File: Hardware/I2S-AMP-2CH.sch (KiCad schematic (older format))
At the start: 21 parts, among them U4 TAS5760MDCAR

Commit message: various fixes
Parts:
- removed C32: 100n, Capacitor_SMD:C_0603_1608Metric_Pad1.08x0.95mm_HandSolder, symbol dsp-amplifier-x4-rescue:Capacitor
- removed C36, C37: 4.7u, Capacitor_SMD:C_0805_2012Metric_Pad1.18x1.45mm_HandSolder, symbol dsp-amplifier-x4-rescue:Capacitor
- removed U4: TAS5760MDCAR, AMPx2 _footprints:HTSSOP-48, symbol dsp-amplifier-x4-rescue:TAS5760MDCAR
- added C32: 470u, Capacitor_THT:CP_Radial_D14.0mm_P5.00mm, symbol Device:CP
- added U?1: TAS5760MDCAR, Package_SO:HTSSOP-32-1EP_6.1x11mm_P0.65mm_EP5.2x11mm_Mask4.11x4.36mm_ThermalVias, symbol tas5760:TAS5760MDCAR
- C25: value 1u -> 100n; Mfr.Nr. GRM188R71C105KE15D -> GRM188R71H104KA93D
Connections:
- net labels added: FREQ, PBTL
- wire segments 107 -> 100
- no-connect marks 14 -> 0

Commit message: started routing
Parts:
- removed C35: 220n, Capacitor_SMD:C_0603_1608Metric_Pad1.08x0.95mm_HandSolder, symbol dsp-amplifier-x4-rescue:Capacitor
- removed C38, C40, C41: 680n, Capacitor_SMD:C_0603_1608Metric_Pad1.08x0.95mm_HandSolder, symbol dsp-amplifier-x4-rescue:Capacitor
- removed L2, L3, L4: 10u, Capacitor_SMD:C_0805_2012Metric_Pad1.18x1.45mm_HandSolder, symbol dsp-amplifier-x4-rescue:Inductor
- added C56: 220n, Capacitor_SMD:C_0603_1608Metric_Pad1.08x0.95mm_HandSolder, symbol Device:C
- added C59, C60, C61: 680n, Capacitor_SMD:C_0603_1608Metric_Pad1.08x0.95mm_HandSolder, symbol Device:C
- added L4, L5, L6: 10u, Inductor_SMD:L_Abracon_ASPI-0630LR, symbol Device:L
- C48: renamed from C26; footprint Capacitor_SMD:C_0603_1608Metric_Pad1.08x0.95mm_HandSolder -> Capacitor_SMD:C_0805_2012Metric_Pad1.18x1.45mm_HandSolder; symbol dsp-amplifier-x4-rescue:Capacitor -> Device:C
- C49: renamed from C27; footprint Capacitor_SMD:C_0603_1608Metric_Pad1.08x0.95mm_HandSolder -> Capacitor_SMD:C_0805_2012Metric_Pad1.18x1.45mm_HandSolder; symbol dsp-amplifier-x4-rescue:Capacitor -> Device:C
- C50: renamed from C30; footprint Capacitor_SMD:C_0603_1608Metric_Pad1.08x0.95mm_HandSolder -> Capacitor_SMD:C_0805_2012Metric_Pad1.18x1.45mm_HandSolder; symbol dsp-amplifier-x4-rescue:Capacitor -> Device:C
- C51: renamed from C25; symbol dsp-amplifier-x4-rescue:Capacitor -> Device:C
- C52: renamed from C31; symbol dsp-amplifier-x4-rescue:Capacitor -> Device:C
- C53: renamed from C32; footprint Capacitor_THT:CP_Radial_D14.0mm_P5.00mm -> Capacitor_THT:CP_Radial_D16.0mm_P7.50mm
- C54: renamed from C34; symbol dsp-amplifier-x4-rescue:Capacitor -> Device:C
- C55: renamed from C29; symbol dsp-amplifier-x4-rescue:Capacitor -> Device:C
- C57: renamed from C33; symbol dsp-amplifier-x4-rescue:Capacitor -> Device:C
- C58: renamed from C39; symbol dsp-amplifier-x4-rescue:Capacitor -> Device:C
- L3: renamed from L1; footprint Capacitor_SMD:C_0805_2012Metric_Pad1.18x1.45mm_HandSolder -> Inductor_SMD:L_Abracon_ASPI-0630LR; symbol dsp-amplifier-x4-rescue:Inductor -> Device:L
- renumbered U?1 to U6
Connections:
- wire segments 100 -> 106

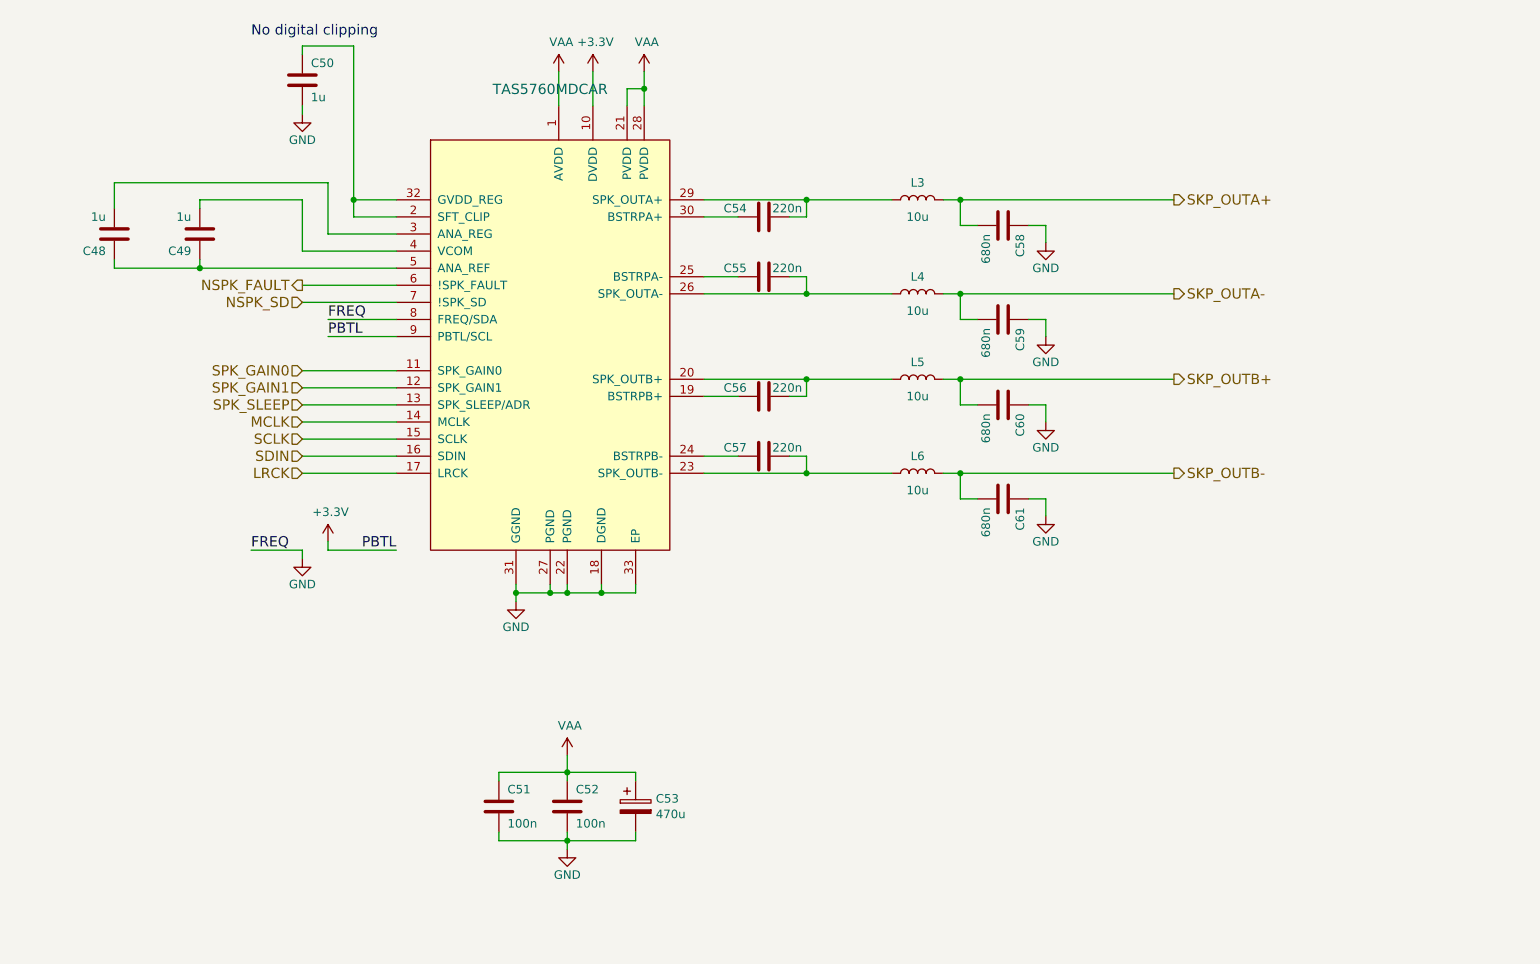
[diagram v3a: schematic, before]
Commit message: bugfixes, made smaller
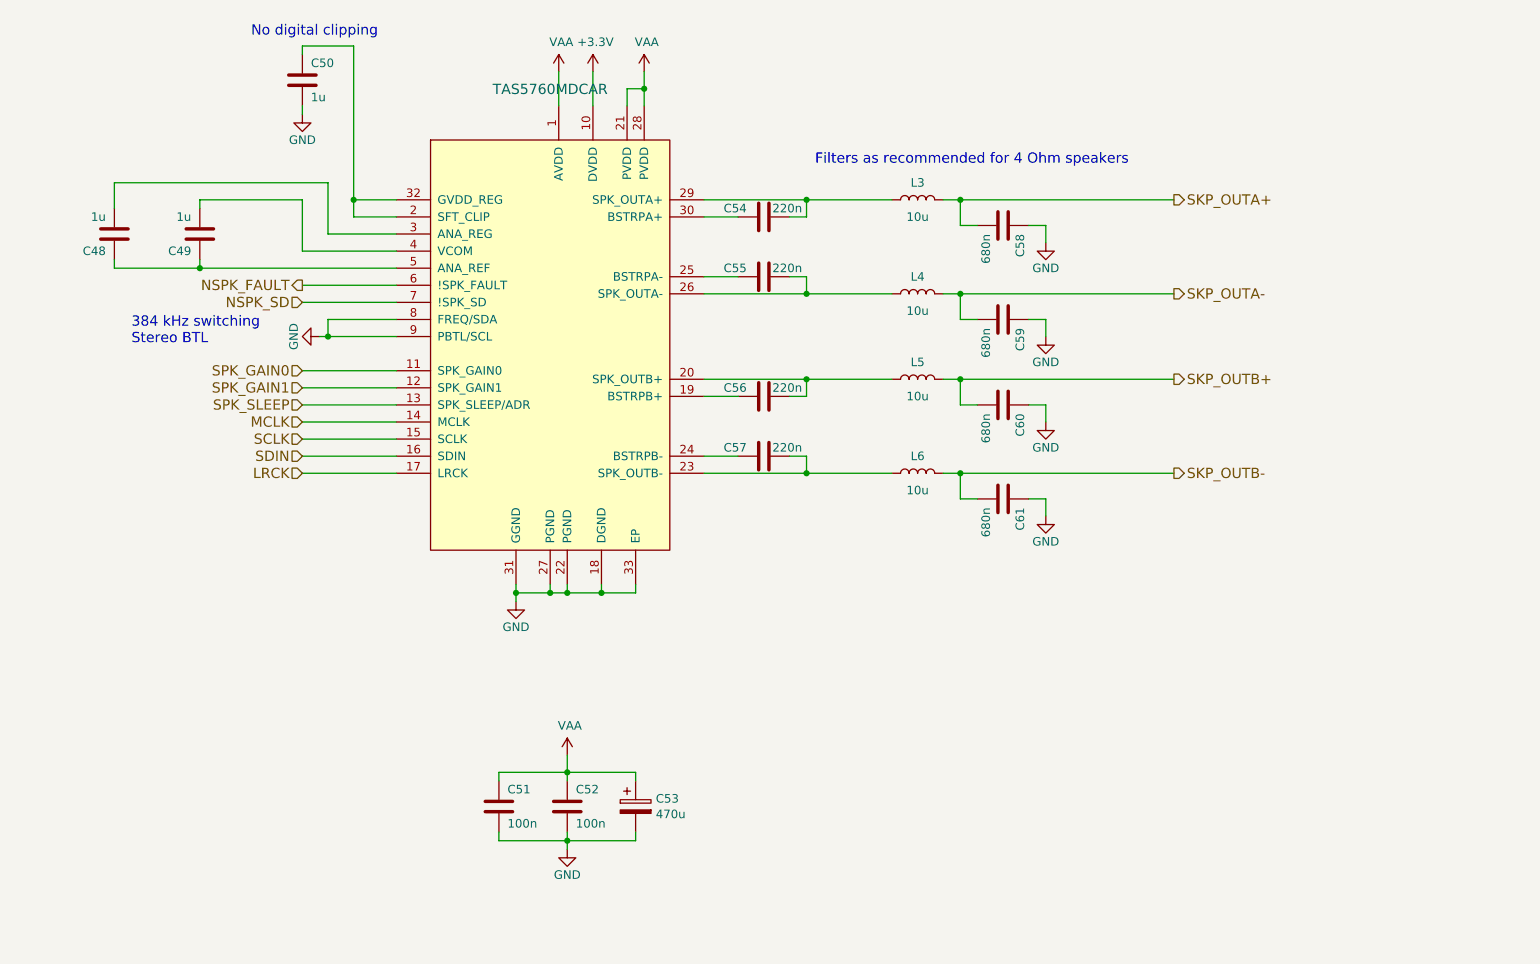
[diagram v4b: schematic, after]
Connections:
- net +3V3: no longer U6.9 (PBTL/SCL)
- net GND: now also U6.9 (PBTL/SCL)
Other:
- note added: "384 kHz switching\nStereo BTL"
- note added: "Filters as recommended for 4 Ohm speakers"
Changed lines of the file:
@@
 	0    -1   -1   0
-$EndComp
-$Comp
-L power:GND #PWR073
-U 1 1 5750BB5F
-P 2950 4450
-AR Path="/5AF9FF80/5750BB5F" Ref="#PWR073"  Part="1"
-AR Path="/608A6138/5750BB5F" Ref="#PWR086"  Part="1"
-F 0 "#PWR086" H 2950 4200 50  0001 C CNN
-F 1 "GND" H 2950 4300 50  0000 C CNN
-F 2 "" H 2950 4450 50  0000 C CNN
-F 3 "" H 2950 4450 50  0000 C CNN
-	1    2950 4450
-	1    0    0    -1
 $EndComp
 Wire Wire Line
@@
 Wire Wire Line
 	4500 5600 4500 5700
-$Comp
-L power:+3.3V #PWR?
-U 1 1 60734777
-P 3100 4350
-AR Path="/60734777" Ref="#PWR?"  Part="1"
-AR Path="/5AF9FF80/60734777" Ref="#PWR074"  Part="1"
-AR Path="/608A6138/60734777" Ref="#PWR087"  Part="1"
-F 0 "#PWR087" H 3100 4200 50  0001 C CNN
-F 1 "+3.3V" H 3115 4523 50  0000 C CNN
-F 2 "" H 3100 4350 50  0001 C CNN
-F 3 "" H 3100 4350 50  0001 C CNN
-	1    3100 4350
-	1    0    0    -1
-$EndComp
 $Comp
 L power:VAA #PWR077
@@
 Wire Wire Line
 	2950 1450 3250 1450
-Text Label 3100 3050 0    60   ~ 0
-FREQ
-Text Label 3100 3150 0    60   ~ 0
-PBTL
 Wire Wire Line
 	3100 3050 3500 3050
-Wire Wire Line
-	3500 3150 3100 3150
-Text Label 2650 4400 0    60   ~ 0
-FREQ
-Text Label 3500 4400 2    60   ~ 0
-PBTL
-Wire Wire Line
-	3500 4400 3100 4400
-Wire Wire Line
-	3100 4350 3100 4400
-Wire Wire Line
-	2950 4450 2950 4400
-Wire Wire Line
-	2950 4400 2650 4400
 $Comp
 L power:+3.3V #PWR?
@@
 Wire Wire Line
 	4100 6050 4100 6100
-$Comp
-L tas5760:TAS5760MDCAR U6
-U 1 1 608A7BF7
-P 4400 3200
-AR Path="/5AF9FF80/608A7BF7" Ref="U6"  Part="1"
-AR Path="/608A6138/608A7BF7" Ref="U7"  Part="1"
-F 0 "U6" H 4400 5150 60  0001 C TNN
-F 1 "TAS5760MDCAR" H 4400 4697 60  0000 C CNN
-F 2 "Package_SO:HTSSOP-32-1EP_6.1x11mm_P0.65mm_EP5.2x11mm_Mask4.11x4.36mm_ThermalVias" H 4300 3100 60  0001 C CNN
-F 3 "" H 4400 3200 60  0000 C CNN
-	1    4400 3200
-	1    0    0    -1
-$EndComp
 Wire Wire Line
 	5300 3950 5900 3950
@@
 	4900 4650 4900 4600
 Connection ~ 4700 4650
+$Comp
+L power:GND #PWR0122
+U 1 1 60B105F1
+P 3050 3150
+AR Path="/5AF9FF80/60B105F1" Ref="#PWR0122"  Part="1"
+AR Path="/608A6138/60B105F1" Ref="#PWR0124"  Part="1"
+F 0 "#PWR0124" H 3050 2900 50  0001 C CNN
+F 1 "GND" H 3050 3000 50  0000 C CNN
+F 2 "" H 3050 3150 50  0000 C CNN
+F 3 "" H 3050 3150 50  0000 C CNN
+	1    3050 3150
+	0    1    1    0
+$EndComp
+$Comp
+L tas5760:TAS5760MDCAR U6
+U 1 1 608A7BF7
+P 4400 3200
+AR Path="/5AF9FF80/608A7BF7" Ref="U6"  Part="1"
+AR Path="/608A6138/608A7BF7" Ref="U7"  Part="1"
+F 0 "U6" H 4400 5150 60  0001 C TNN
+F 1 "TAS5760MDCAR" H 4400 4697 60  0000 C CNN
+F 2 "Package_SO:HTSSOP-32-1EP_6.1x11mm_P0.65mm_EP5.2x11mm_Mask4.11x4.36mm_ThermalVias" H 4300 3100 60  0001 C CNN
+F 3 "" H 4400 3200 60  0000 C CNN
+	1    4400 3200
+	1    0    0    -1
+$EndComp
+Wire Wire Line
+	3050 3150 3100 3150
+Wire Wire Line
+	3100 3050 3100 3150
+Connection ~ 3100 3150
+Wire Wire Line
+	3100 3150 3500 3150
+Text Notes 5950 2150 0    60   ~ 0
+Filters as recommended for 4 Ohm speakers
+Text Notes 1950 3200 0    60   ~ 0
+384 kHz switching\nStereo BTL
 $EndSCHEMATC

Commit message: style fixes, spi/i2c
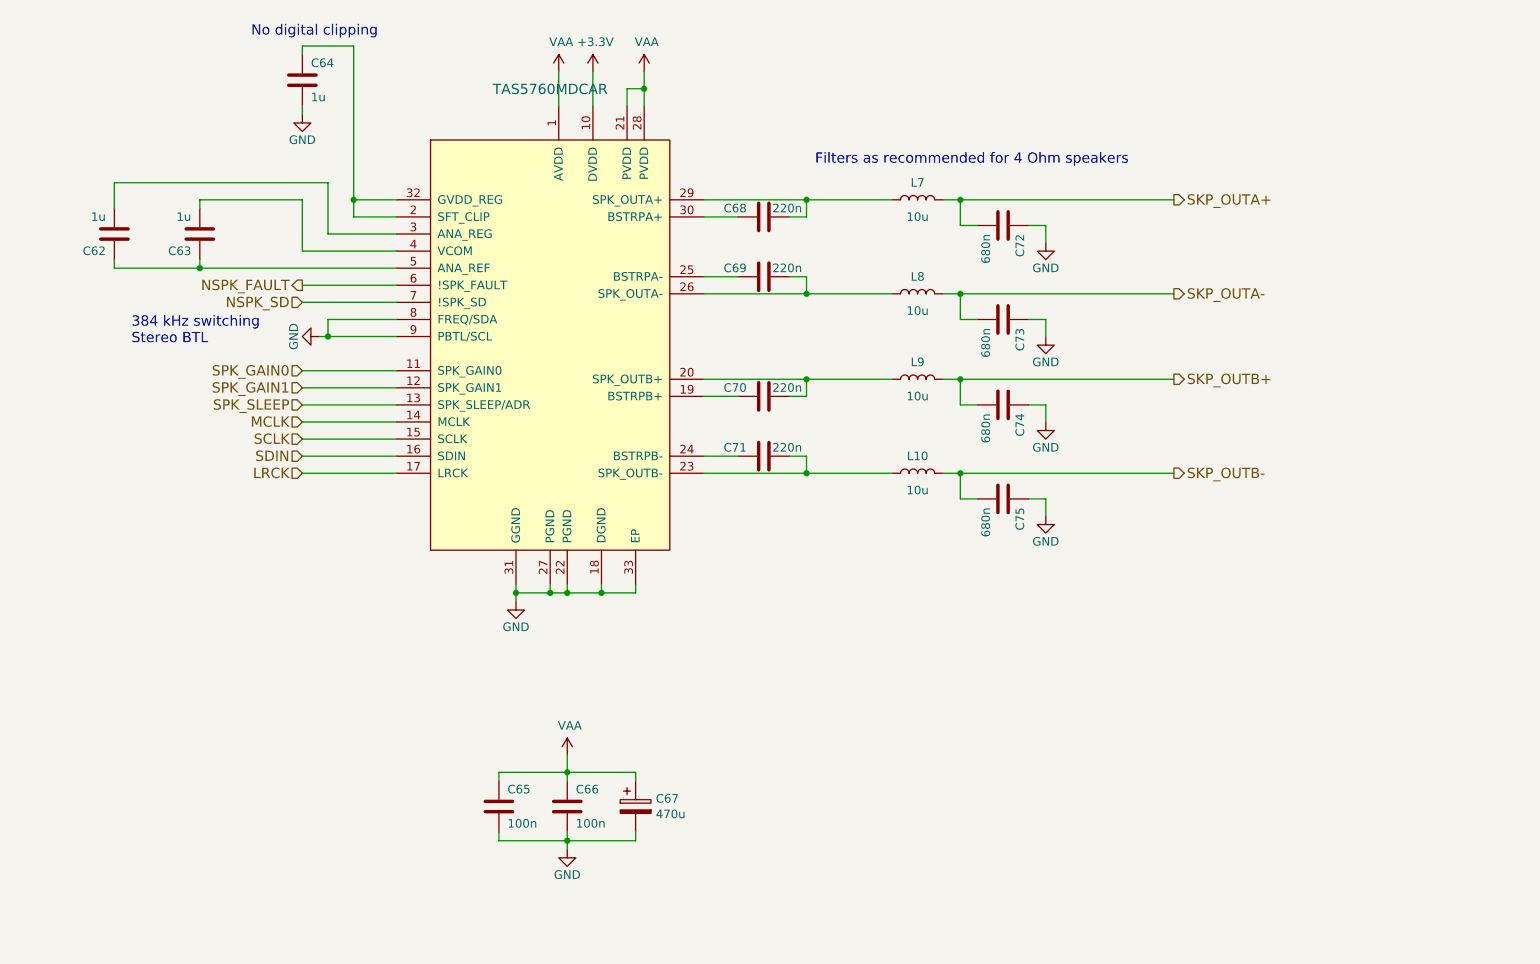
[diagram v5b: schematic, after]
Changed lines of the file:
@@
 AR Path="/5AF9FF80/574C11BE" Ref="C50"  Part="1"
 AR Path="/608A6138/574C11BE" Ref="C64"  Part="1"
-F 0 "C50" H 3000 1750 50  0000 L CNN
+F 0 "C64" H 3000 1750 50  0000 L CNN
 F 1 "1u" H 3000 1550 50  0000 L CNN
 F 2 "Capacitor_SMD:C_0805_2012Metric_Pad1.18x1.45mm_HandSolder" V 2650 1790 50  0001 C CNN
@@
 AR Path="/5AF9FF80/5B067CFE" Ref="C49"  Part="1"
 AR Path="/608A6138/5B067CFE" Ref="C63"  Part="1"
-F 0 "C49" H 2400 2650 50  0000 L CNN
+F 0 "C63" H 2400 2650 50  0000 L CNN
 F 1 "1u" H 2400 2450 50  0000 L CNN
 F 2 "Capacitor_SMD:C_0805_2012Metric_Pad1.18x1.45mm_HandSolder" V 2050 2690 50  0001 C CNN
@@
 AR Path="/5AF9FF80/5B067CFF" Ref="C48"  Part="1"
 AR Path="/608A6138/5B067CFF" Ref="C62"  Part="1"
-F 0 "C48" H 1900 2650 50  0000 L CNN
+F 0 "C62" H 1900 2650 50  0000 L CNN
 F 1 "1u" H 1900 2450 50  0000 L CNN
 F 2 "Capacitor_SMD:C_0805_2012Metric_Pad1.18x1.45mm_HandSolder" V 1550 2690 50  0001 C CNN
@@
 AR Path="/5AF9FF80/574C26C6" Ref="C52"  Part="1"
 AR Path="/608A6138/574C26C6" Ref="C66"  Part="1"
-F 0 "C52" H 4550 6000 50  0000 L CNN
+F 0 "C66" H 4550 6000 50  0000 L CNN
 F 1 "100n" H 4550 5800 50  0000 L CNN
 F 2 "Capacitor_SMD:C_0603_1608Metric_Pad1.08x0.95mm_HandSolder" V 4200 6040 50  0001 C CNN
@@
 AR Path="/5AF9FF80/5B067D0D" Ref="C57"  Part="1"
 AR Path="/608A6138/5B067D0D" Ref="C71"  Part="1"
-F 0 "C57" V 5700 3950 50  0000 L CNN
+F 0 "C71" V 5700 3950 50  0000 L CNN
 F 1 "220n" V 5700 3800 50  0000 R CNN
 F 2 "Capacitor_SMD:C_0603_1608Metric_Pad1.08x0.95mm_HandSolder" V 5350 3990 50  0001 C CNN
@@
 AR Path="/5AF9FF80/5B067D11" Ref="C55"  Part="1"
 AR Path="/608A6138/5B067D11" Ref="C69"  Part="1"
-F 0 "C55" V 5700 2900 50  0000 L CNN
+F 0 "C69" V 5700 2900 50  0000 L CNN
 F 1 "220n" V 5700 2750 50  0000 R CNN
 F 2 "Capacitor_SMD:C_0603_1608Metric_Pad1.08x0.95mm_HandSolder" V 5350 2940 50  0001 C CNN
@@
 AR Path="/5AF9FF80/5B067D13" Ref="C54"  Part="1"
 AR Path="/608A6138/5B067D13" Ref="C68"  Part="1"
-F 0 "C54" V 5700 2550 50  0000 L CNN
+F 0 "C68" V 5700 2550 50  0000 L CNN
 F 1 "220n" V 5700 2400 50  0000 R CNN
 F 2 "Capacitor_SMD:C_0603_1608Metric_Pad1.08x0.95mm_HandSolder" V 5350 2590 50  0001 C CNN
@@
 AR Path="/5AF9FF80/6097B2F1" Ref="C53"  Part="1"
 AR Path="/608A6138/6097B2F1" Ref="C67"  Part="1"
-F 0 "C53" H 5018 5946 50  0000 L CNN
+F 0 "C67" H 5018 5946 50  0000 L CNN
 F 1 "470u" H 5018 5855 50  0000 L CNN
 F 2 "Capacitor_THT:CP_Radial_D16.0mm_P7.50mm" H 4938 5750 50  0001 C CNN
@@
 AR Path="/5AF9FF80/60988667" Ref="C51"  Part="1"
 AR Path="/608A6138/60988667" Ref="C65"  Part="1"
-F 0 "C51" H 4150 6000 50  0000 L CNN
+F 0 "C65" H 4150 6000 50  0000 L CNN
 F 1 "100n" H 4150 5800 50  0000 L CNN
 F 2 "Capacitor_SMD:C_0603_1608Metric_Pad1.08x0.95mm_HandSolder" V 3800 6040 50  0001 C CNN
@@
 AR Path="/5AF9FF80/5B067D14" Ref="L3"  Part="1"
 AR Path="/608A6138/5B067D14" Ref="L7"  Part="1"
-F 0 "L3" V 6650 2350 50  0000 C CNN
+F 0 "L7" V 6650 2350 50  0000 C CNN
 F 1 "10u" V 6450 2350 50  0000 C CNN
 F 2 "Inductor_SMD:L_Abracon_ASPI-0630LR" H 6550 2350 50  0001 C CNN
@@
 AR Path="/5AF9FF80/60D816DE" Ref="L4"  Part="1"
 AR Path="/608A6138/60D816DE" Ref="L8"  Part="1"
-F 0 "L4" V 6650 2900 50  0000 C CNN
+F 0 "L8" V 6650 2900 50  0000 C CNN
 F 1 "10u" V 6450 2900 50  0000 C CNN
 F 2 "Inductor_SMD:L_Abracon_ASPI-0630LR" H 6550 2900 50  0001 C CNN
@@
 AR Path="/5AF9FF80/60D87D8D" Ref="L5"  Part="1"
 AR Path="/608A6138/60D87D8D" Ref="L9"  Part="1"
-F 0 "L5" V 6650 3400 50  0000 C CNN
+F 0 "L9" V 6650 3400 50  0000 C CNN
 F 1 "10u" V 6450 3400 50  0000 C CNN
 F 2 "Inductor_SMD:L_Abracon_ASPI-0630LR" H 6550 3400 50  0001 C CNN
@@
 AR Path="/5AF9FF80/60D87DA0" Ref="L6"  Part="1"
 AR Path="/608A6138/60D87DA0" Ref="L10"  Part="1"
-F 0 "L6" V 6650 3950 50  0000 C CNN
+F 0 "L10" V 6650 3950 50  0000 C CNN
 F 1 "10u" V 6450 3950 50  0000 C CNN
 F 2 "Inductor_SMD:L_Abracon_ASPI-0630LR" H 6550 3950 50  0001 C CNN
@@
 AR Path="/5AF9FF80/5B067D19" Ref="C58"  Part="1"
 AR Path="/608A6138/5B067D19" Ref="C72"  Part="1"
-F 0 "C58" H 7100 2600 50  0000 L CNN
+F 0 "C72" H 7100 2600 50  0000 L CNN
 F 1 "680n" H 7100 2400 50  0000 L CNN
 F 2 "Capacitor_SMD:C_0603_1608Metric_Pad1.08x0.95mm_HandSolder" V 6750 2640 50  0001 C CNN
@@
 AR Path="/5AF9FF80/60D9BA43" Ref="C59"  Part="1"
 AR Path="/608A6138/60D9BA43" Ref="C73"  Part="1"
-F 0 "C59" H 7100 3150 50  0000 L CNN
+F 0 "C73" H 7100 3150 50  0000 L CNN
 F 1 "680n" H 7100 2950 50  0000 L CNN
 F 2 "Capacitor_SMD:C_0603_1608Metric_Pad1.08x0.95mm_HandSolder" V 6750 3190 50  0001 C CNN
@@
 AR Path="/5AF9FF80/60D9DAD3" Ref="C60"  Part="1"
 AR Path="/608A6138/60D9DAD3" Ref="C74"  Part="1"
-F 0 "C60" H 7100 3650 50  0000 L CNN
+F 0 "C74" H 7100 3650 50  0000 L CNN
 F 1 "680n" H 7100 3450 50  0000 L CNN
 F 2 "Capacitor_SMD:C_0603_1608Metric_Pad1.08x0.95mm_HandSolder" V 6750 3690 50  0001 C CNN
@@
 AR Path="/5AF9FF80/60D9FB44" Ref="C61"  Part="1"
 AR Path="/608A6138/60D9FB44" Ref="C75"  Part="1"
-F 0 "C61" H 7100 4200 50  0000 L CNN
+F 0 "C75" H 7100 4200 50  0000 L CNN
 F 1 "680n" H 7100 4000 50  0000 L CNN
 F 2 "Capacitor_SMD:C_0603_1608Metric_Pad1.08x0.95mm_HandSolder" V 6750 4240 50  0001 C CNN
@@
 AR Path="/5AF9FF80/60C136E8" Ref="C56"  Part="1"
 AR Path="/608A6138/60C136E8" Ref="C70"  Part="1"
-F 0 "C56" V 5700 3600 50  0000 L CNN
+F 0 "C70" V 5700 3600 50  0000 L CNN
 F 1 "220n" V 5700 3450 50  0000 R CNN
 F 2 "Capacitor_SMD:C_0603_1608Metric_Pad1.08x0.95mm_HandSolder" V 5350 3640 50  0001 C CNN
@@
 AR Path="/5AF9FF80/608A7BF7" Ref="U6"  Part="1"
 AR Path="/608A6138/608A7BF7" Ref="U7"  Part="1"
-F 0 "U6" H 4400 5150 60  0001 C TNN
+F 0 "U7" H 4400 5150 60  0001 C TNN
 F 1 "TAS5760MDCAR" H 4400 4697 60  0000 C CNN
 F 2 "Package_SO:HTSSOP-32-1EP_6.1x11mm_P0.65mm_EP5.2x11mm_Mask4.11x4.36mm_ThermalVias" H 4300 3100 60  0001 C CNN
